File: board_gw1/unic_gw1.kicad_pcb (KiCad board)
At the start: 4 copper layers, 49.5 x 15.2 mm, 112 parts, among them Q1 2N7002, Q10 2N7002, Q11 2N7002, Q12 2N7002, Q13 2N7002, Q14 2N7002, Q15 2N7002, Q16 2N7002, Q17 2N7002, Q18 2N7002, Q19 2N7002, Q2 2N7002, Q20 2N7002, Q21 2N7002, Q22 2N7002, Q23 2N7002, Q24 2N7002, Q25 2N7002, Q26 2N7002, Q27 2N7002, Q28 2N7002, Q29 2N7002, Q3 2N7002, Q30 2N7002, Q31 2N7002, Q32 2N7002, Q33 2N7002, Q34 2N7002, Q35 2N7002, Q36 2N7002, Q37 2N7002, Q38 2N7002, Q39 2N7002, Q4 2N7002, Q40 2N7002, Q5 2N7002, Q6 2N7002, Q7 2N7002, Q8 2N7002, Q9 2N7002, U1 GW1N-LV9QN88C6_I5_, U2 LM3480-3.3, U3 AP2202K-ADJ, U4 APS6404L-3SQR-ZR, U6 AP62150Z6, U7 W25Q16JVUXIQ, X1 27MHz

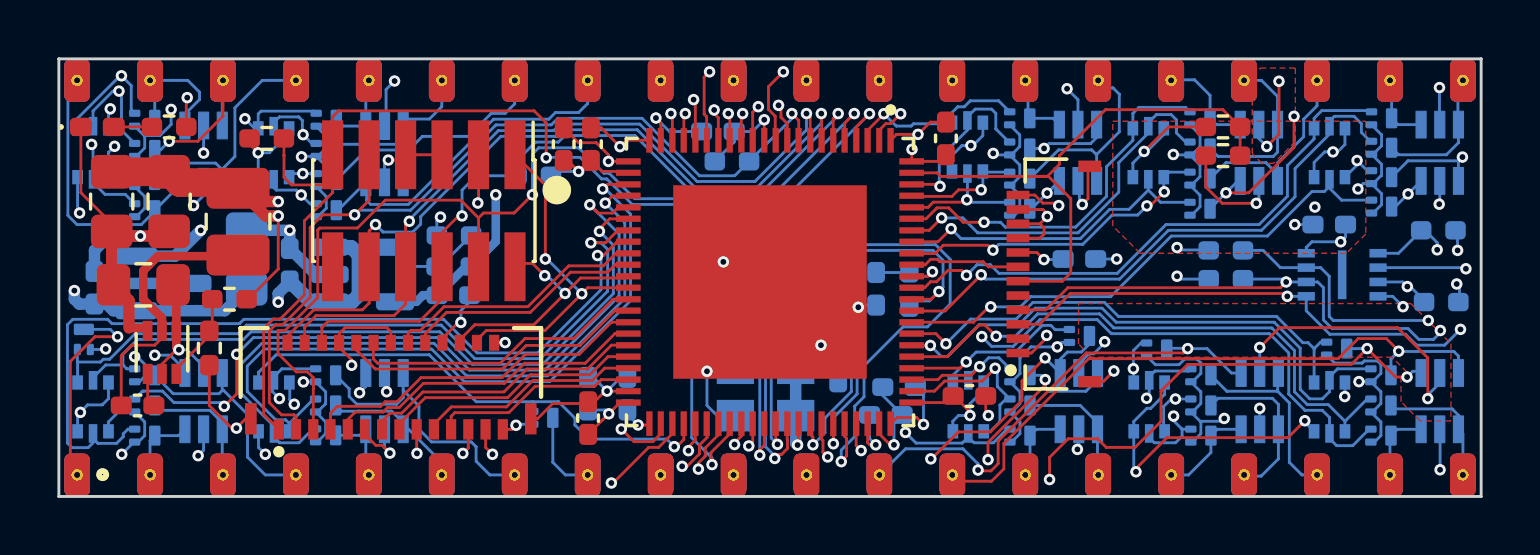
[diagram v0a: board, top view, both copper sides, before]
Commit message: Ready to roll with DEVEL board!
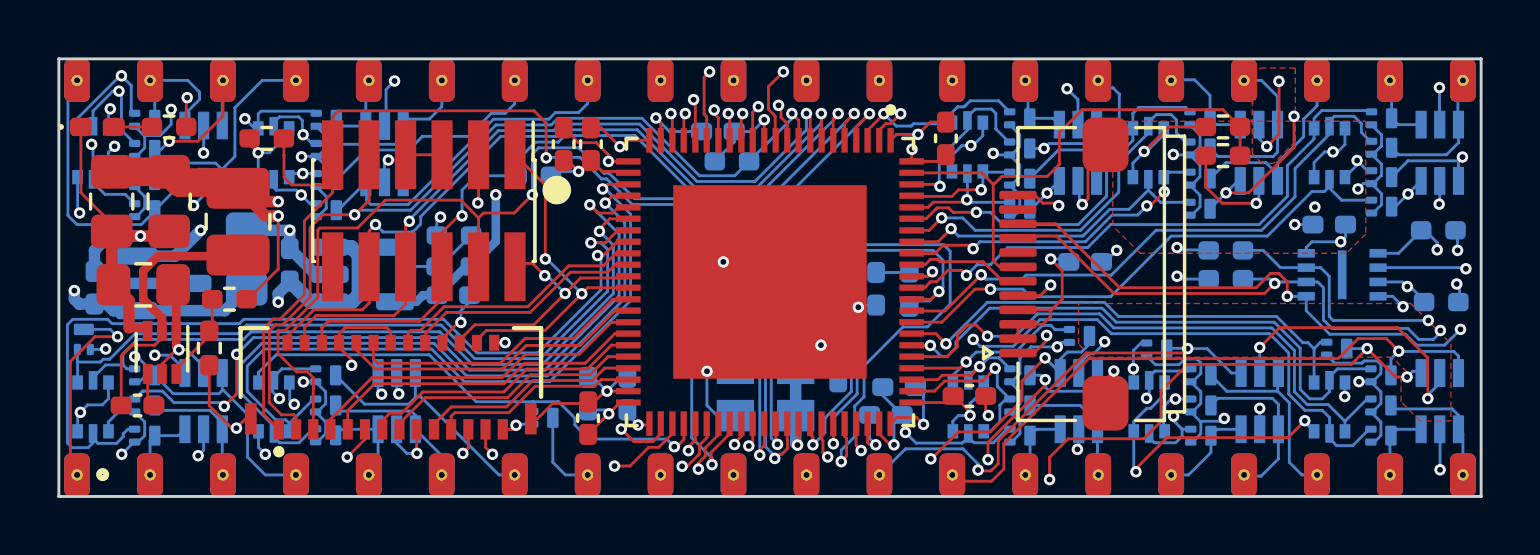
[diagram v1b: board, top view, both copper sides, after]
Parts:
- J_DISPLAY1: footprint UNIC:HRS_FH19C-12S-0.5SH_05_ -> UNIC:CF31121D0R0-05-NH
- moved D2 0.42 mm to (136.2, 99.5)
- moved C16 0.22 mm to (160.2, 94.7), turned to 0 degrees
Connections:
- J_DISPLAY1 pad 10: +3V3 -> /SPI_MOSI_IO0
- J_DISPLAY1 pad 11: +3V3 -> unconnected-(J_DISPLAY1-Pin_11-Pad11)
- J_DISPLAY1 pad 2: unconnected-(J_DISPLAY1-Pin_2-Pad2) -> +3V3
- J_DISPLAY1 pad 3: /SPI_MOSI_IO0 -> +3V3
- J_DISPLAY1 pad 4: /SPI_CLK -> +3V3
- J_DISPLAY1 pad 5: unconnected-(J_DISPLAY1-Pin_5-Pad5) -> GND
- J_DISPLAY1 pad 6: /LCD_RST_N -> /LCD_CS_N
- J_DISPLAY1 pad 7: /LCD_CS_N -> /LCD_RST_N
- J_DISPLAY1 pad 8: GND -> unconnected-(J_DISPLAY1-Pin_8-Pad8)
- J_DISPLAY1 pad 9: +3V3 -> /SPI_CLK
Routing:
- net /LCD_RST_N: track 20.3 -> 18.2 mm
- net /PIN8: track 13.5 -> 12.1 mm
- net +3V3: track 74.9 -> 76.2 mm, vias 29 -> 28
- net /SPI_MOSI_IO0: track 52.3 -> 53.5 mm
- net /PIN7: track 9.75 -> 8.73 mm
- net GND: track 81.8 -> 82.5 mm, vias 37 -> 38
- net LINE: track 45.9 -> 46.4 mm
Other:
- board text added: "Standard DIP40 top"
